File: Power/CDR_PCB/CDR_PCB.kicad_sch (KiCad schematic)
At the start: 16 parts, among them IC1 TEENSY_4.1, J1 +5V, J2 +3V3, U1 INA226, U2 BNO055, U3 DPS310XTSA1, U4 GNSS

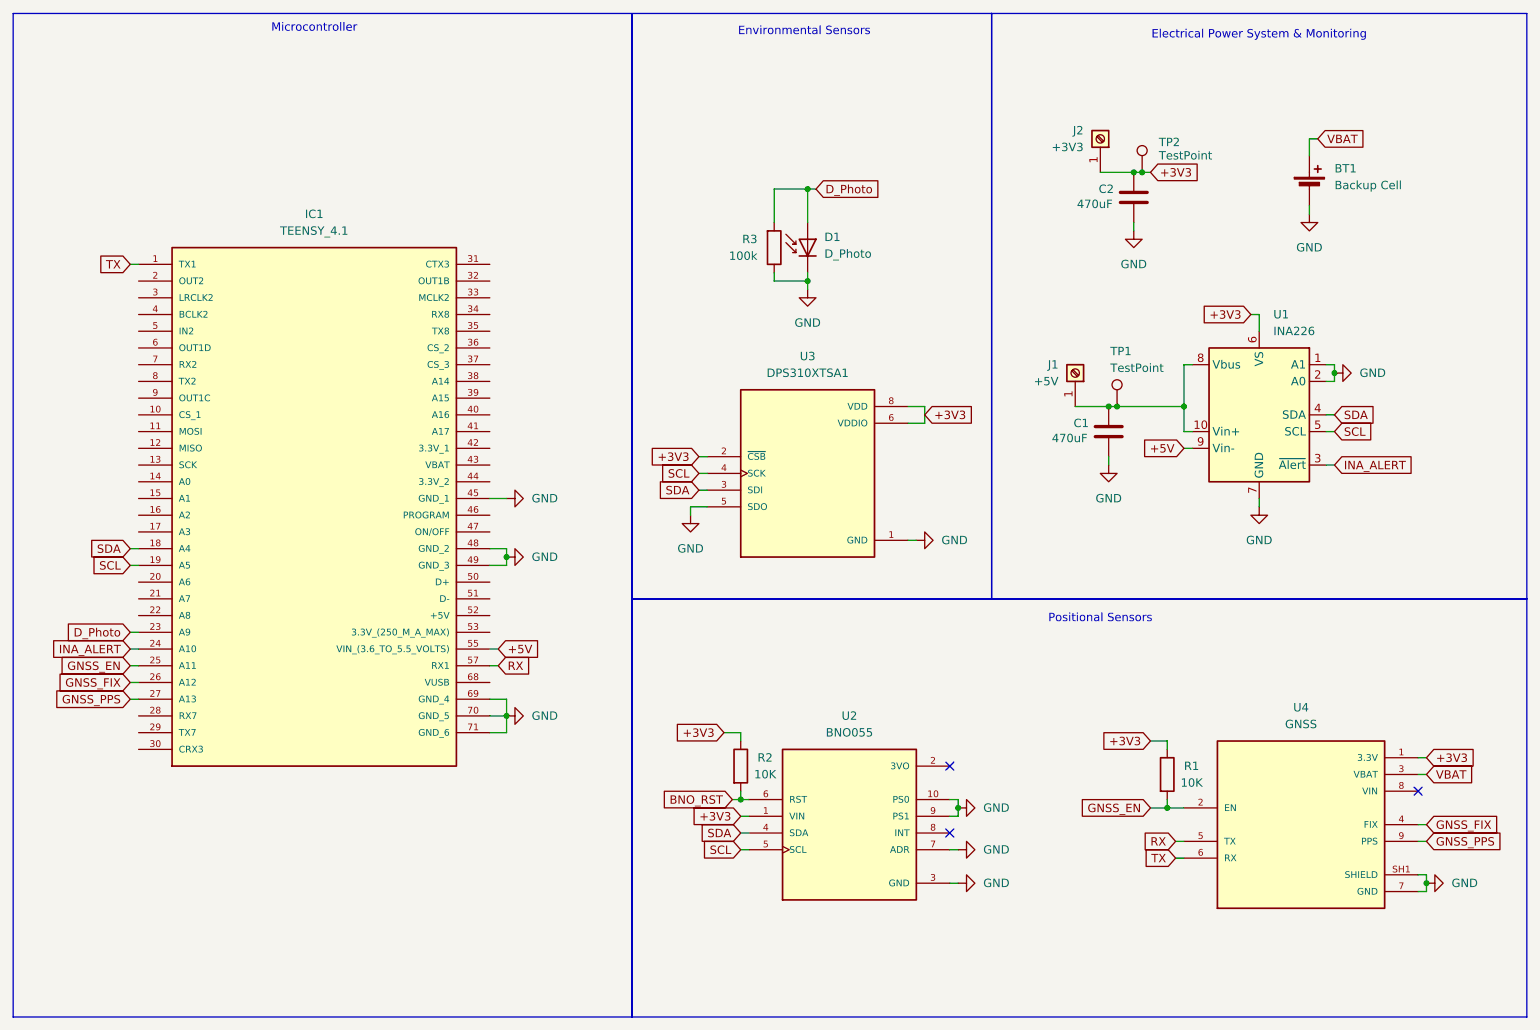
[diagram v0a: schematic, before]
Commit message: Finalised PCB Schematic with missing components
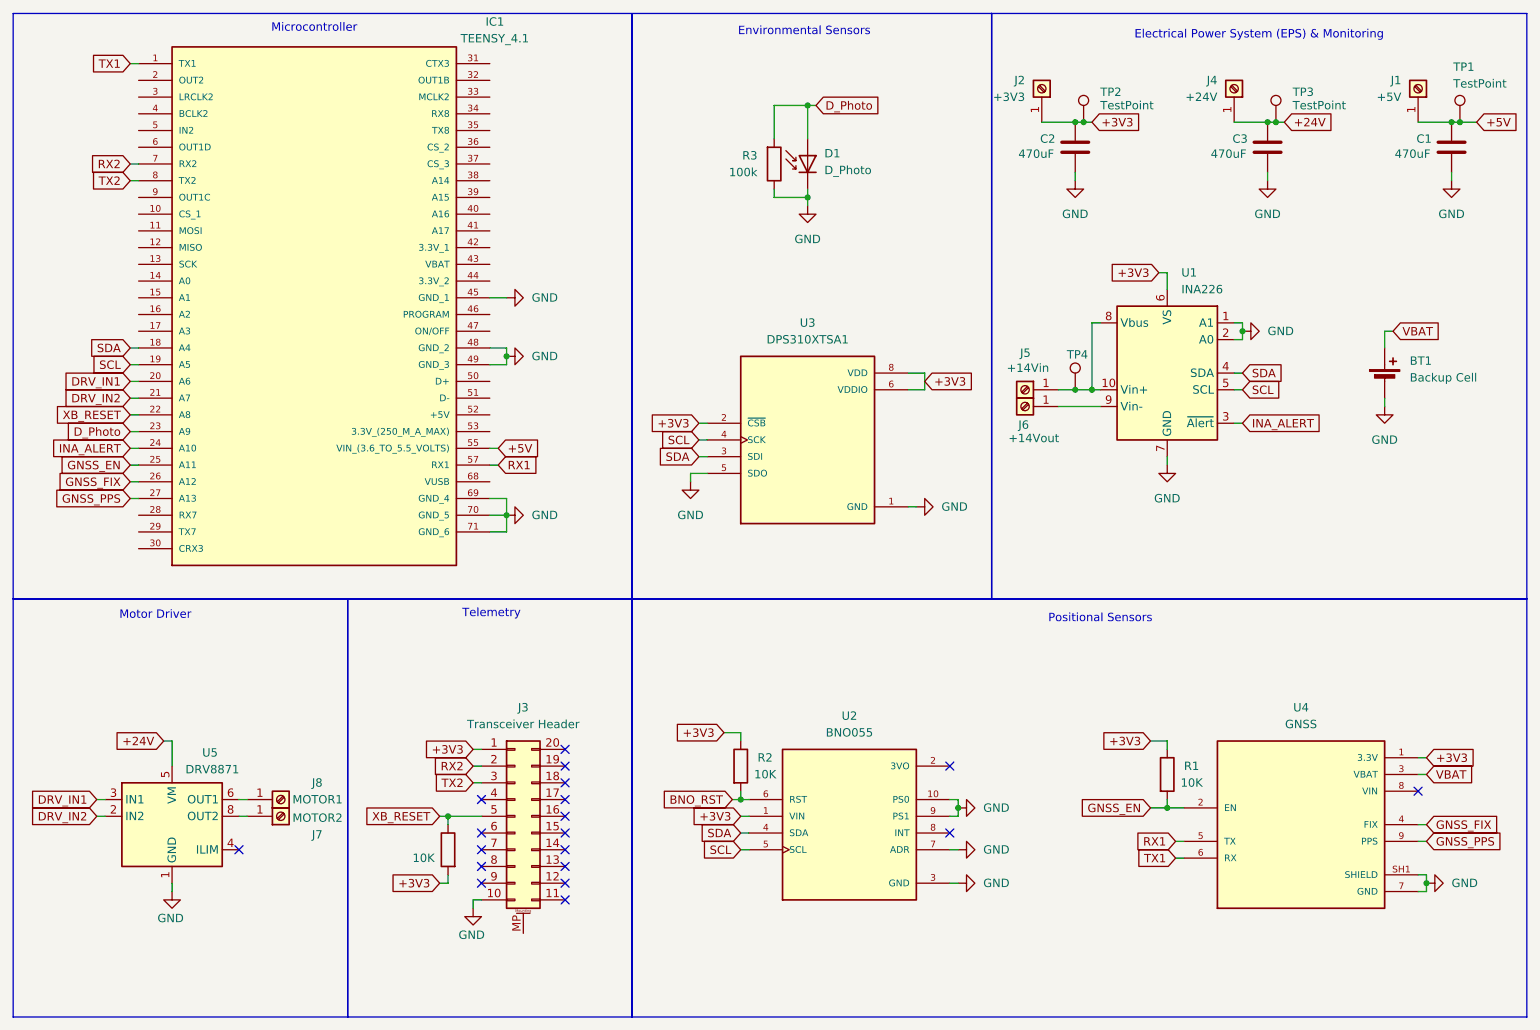
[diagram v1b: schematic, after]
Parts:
- added C3: 470uF, Capacitor_THT:CP_Radial_D8.0mm_P3.50mm, symbol Device:C
- added J3: Transceiver Header, Connector_PinHeader_2.54mm:PinHeader_1x05_P2.54mm_Vertical, symbol Connector_Generic_MountingPin:Conn_02x10_Counter_Clockwise_MountingPin
- added J4: +24V, Connector_PinHeader_2.54mm:PinHeader_1x01_P2.54mm_Vertical, symbol Connector:Screw_Terminal_01x01
- added J5: +14Vin, Connector_PinHeader_2.54mm:PinHeader_1x01_P2.54mm_Vertical, symbol Connector:Screw_Terminal_01x01
- added J6: +14Vout, Connector_PinHeader_2.54mm:PinHeader_1x01_P2.54mm_Vertical, symbol Connector:Screw_Terminal_01x01
- added J7: MOTOR2, Connector_PinHeader_2.54mm:PinHeader_1x01_P2.54mm_Vertical, symbol Connector:Screw_Terminal_01x01
- added J8: MOTOR1, Connector_PinHeader_2.54mm:PinHeader_1x01_P2.54mm_Vertical, symbol Connector:Screw_Terminal_01x01
- added R4: 10K, Resistor_THT:R_Axial_DIN0207_L6.3mm_D2.5mm_P7.62mm_Horizontal, symbol Device:R
- added TP3, TP4: TestPoint, TestPoint:TestPoint_Loop_D2.50mm_Drill1.0mm, symbol Connector:TestPoint
- added U5: DRV8871, Package_SO:Texas_HTSOP-8-1EP_3.9x4.9mm_P1.27mm_EP2.95x4.9mm_Mask2.4x3.1mm_ThermalVias, symbol Driver_Motor:DRV8871DDA
- BT1: footprint (none) -> Battery:BatteryHolder_Multicomp_BC-2001_1x2032
- U2: footprint 2472:MODULE_2472 -> BNO055:MODULE_2472
- U4: footprint 746:XCVR_746 -> GNSS:XCVR_746
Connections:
- net +3V3: now also J3.1 (Pin_1), R4.2
- net +5V: now also C1.1, J1.1 (Pin_1), TP1.1; no longer U1.9 (Vin-)
- net GND: now also C3.2, J3.10 (Pin_10), U5.1 (GND), U5.7 (GND), U5.9 (GND)
- net DRV_IN1: now reaches IC1.20 (A6)
- net DRV_IN1: now also U5.3 (IN1)
- net DRV_IN2: now reaches IC1.21 (A7)
- net DRV_IN2: now also U5.2 (IN2)
- net XB_RESET: now reaches IC1.22 (A8)
- net XB_RESET: now also J3.5 (Pin_5), R4.1
- net RX2: now reaches IC1.7 (RX2)
- net RX2: now also J3.2 (Pin_2)
- net TX2: now reaches IC1.8 (TX2)
- net TX2: now also J3.3 (Pin_3)
- net RX renamed RX1
- net TX renamed TX1
- new net: J5.1 (Pin_1), TP4.1, U1.10 (Vin+), U1.8 (Vbus)
- new net: J6.1 (Pin_1), U1.9 (Vin-)
- new net: J8.1 (Pin_1), U5.6 (OUT1)
- new net: J7.1 (Pin_1), U5.8 (OUT2)
- new net +24V: C3.1, J4.1 (Pin_1), TP3.1, U5.5 (VM)
- no-connect marks 3 -> 19
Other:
- note added: "Electrical Power System (EPS) & Monitoring"
- note added: "Motor Driver"
- note added: "Telemetry"
- note removed: "Electrical Power System & Monitoring"
- moved on the sheet: BT1, C1, C2, D1, IC1, J1, J2, R3, TP1, TP2, U1, U3
